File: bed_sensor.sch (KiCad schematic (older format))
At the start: 30 parts, among them J1 Conn_01x02, J4 Conn_01x02, Q1 2N2219, Q2 BSS138, Q3 BSS138, SW1 SW_SPST, U1 MIC5205-3.3, U2 MPU-9250, U3 TXB0104D, U4 LTC3525-5, U5 CFAH0802D-YYH-JP

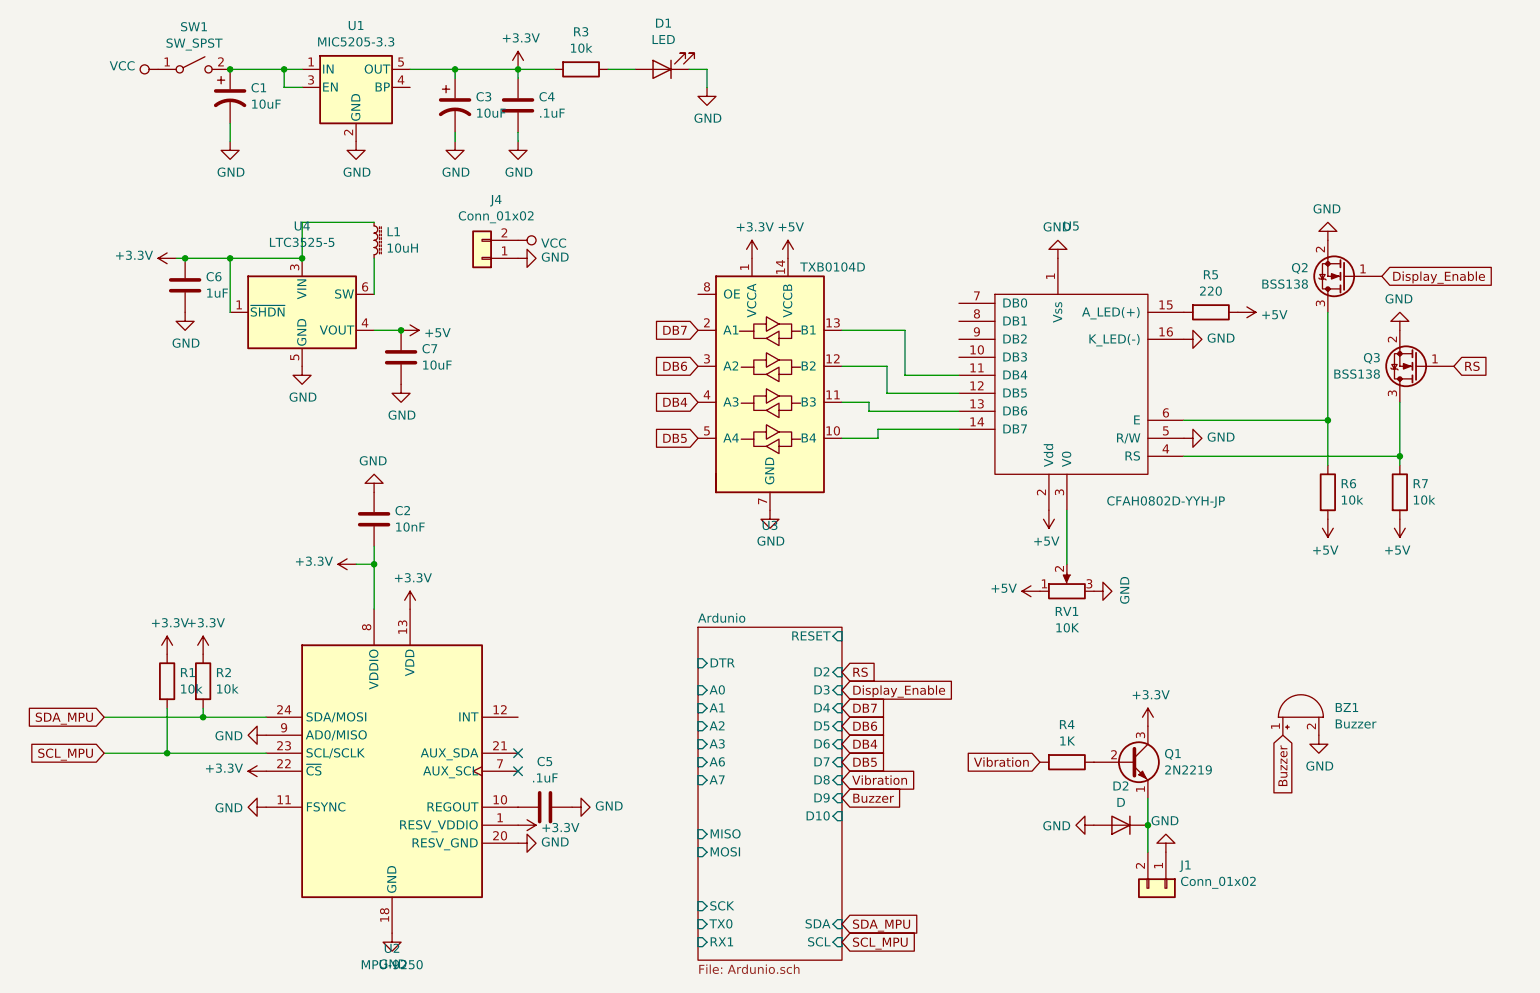
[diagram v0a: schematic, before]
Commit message: updated design
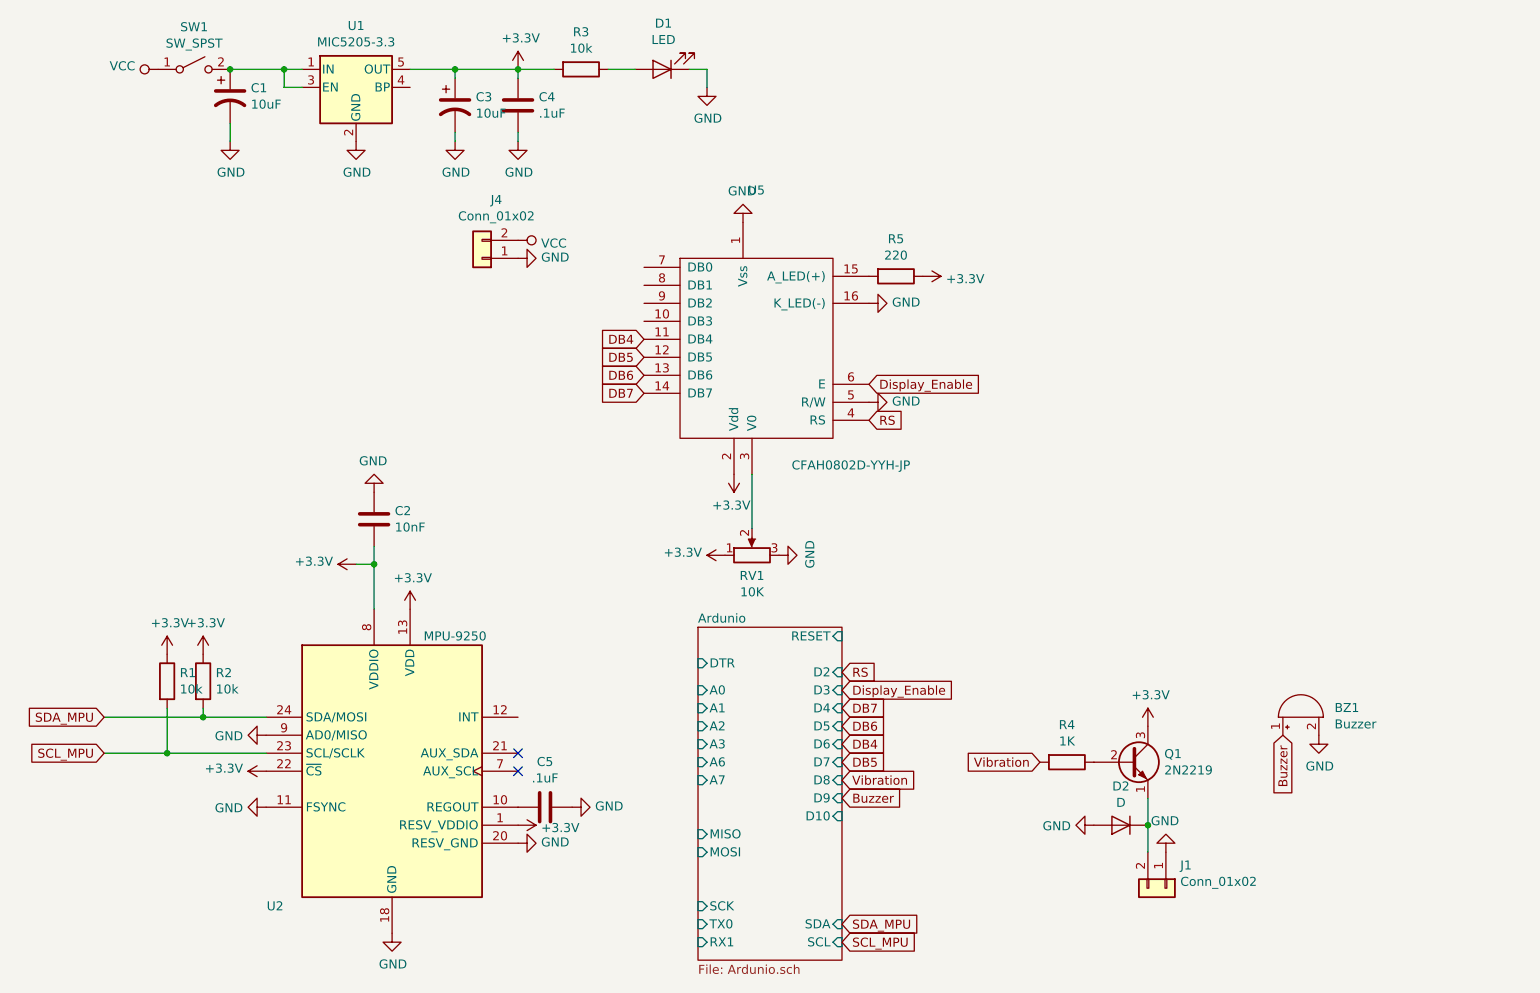
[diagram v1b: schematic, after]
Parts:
- removed C6: 1uF, Capacitor_SMD:C_0603_1608Metric, symbol Device:C
- removed C7: 10uF, Capacitor_SMD:C_0603_1608Metric, symbol Device:C
- removed L1: 10uH, Inductors_SMD:L_Taiyo-Yuden_NR-40xx, symbol Device:L_Core_Ferrite_Small
- removed Q2, Q3: BSS138, Package_TO_SOT_SMD:SOT-23, symbol Transistor_FET:BSS138
- removed R6, R7: 10k, Resistor_SMD:R_0805_2012Metric, symbol Device:R
- removed U3: TXB0104D, Package_SO:SOIC-14_3.9x8.7mm_P1.27mm, symbol Logic_LevelTranslator:TXB0104D
- removed U4: LTC3525-5, Package_TO_SOT_SMD:SOT-363_SC-70-6, symbol Regulator_Switching:LTC3525-5
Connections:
- net +5V is gone; now on net +3V3: R5.1, RV1.1, U5.2 (Vdd)
- net DB4: now also U5.11 (DB4)
- net DB5: now also U5.12 (DB5)
- net DB6: now also U5.13 (DB6)
- net DB7: now also U5.14 (DB7)
- net Display_Enable: now also U5.6 (E)
- net RS: now also U5.4 (RS)
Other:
- moved on the sheet: R5, RV1, U5

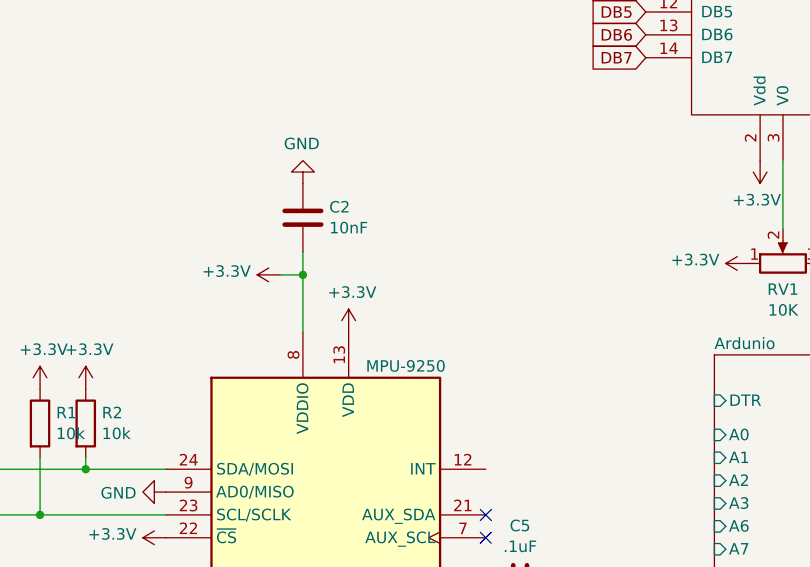
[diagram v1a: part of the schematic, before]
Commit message: updated pcb layout
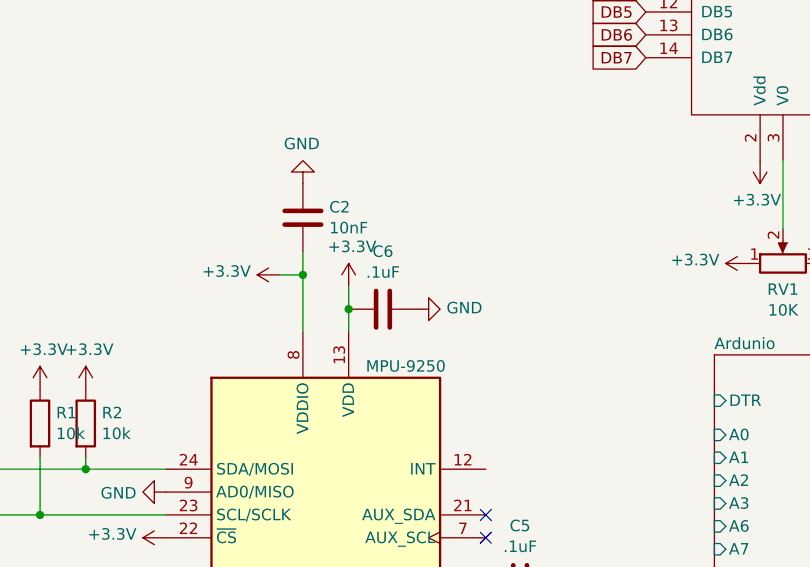
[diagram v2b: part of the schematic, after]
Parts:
- added C6: .1uF, Capacitor_SMD:C_0603_1608Metric, symbol Device:C
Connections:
- net +3V3: now also C6.2
- net GND: now also C6.1
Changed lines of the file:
@@
 L power:+3.3V #PWR0134
 U 1 1 5B151EBC
-P 2950 4150
-F 0 "#PWR0134" H 2950 4000 50  0001 C CNN
-F 1 "+3.3V" H 2965 4323 50  0000 C CNN
-F 2 "" H 2950 4150 50  0001 C CNN
-F 3 "" H 2950 4150 50  0001 C CNN
-	1    2950 4150
+P 2950 3950
+F 0 "#PWR0134" H 2950 3800 50  0001 C CNN
+F 1 "+3.3V" H 2965 4123 50  0000 C CNN
+F 2 "" H 2950 3950 50  0001 C CNN
+F 3 "" H 2950 3950 50  0001 C CNN
+	1    2950 3950
 	1    0    0    -1
 $EndComp
@@
 	0    -1   -1   0
 $EndComp
+$Comp
+L Device:C C6
+U 1 1 5B20EB30
+P 3100 4050
+F 0 "C6" V 2848 4050 50  0000 C CNN
+F 1 ".1uF" V 2939 4050 50  0000 C CNN
+F 2 "Capacitor_SMD:C_0603_1608Metric" H 3138 3900 50  0001 C CNN
+F 3 "~" H 3100 4050 50  0001 C CNN
+	1    3100 4050
+	0    1    1    0
+$EndComp
+$Comp
+L power:GND #PWR0119
+U 1 1 5B20EC20
+P 3250 4050
+F 0 "#PWR0119" H 3250 3800 50  0001 C CNN
+F 1 "GND" V 3255 3922 50  0000 R CNN
+F 2 "" H 3250 4050 50  0001 C CNN
+F 3 "" H 3250 4050 50  0001 C CNN
+	1    3250 4050
+	0    -1   -1   0
+$EndComp
+Wire Wire Line
+	2950 4150 2950 4050
+Connection ~ 2950 4050
+Wire Wire Line
+	2950 4050 2950 3950
 $EndSCHEMATC
